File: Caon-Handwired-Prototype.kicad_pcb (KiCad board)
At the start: 6 copper layers, 27 parts, among them SW4 EC11 ENCODER 1, SW8 EC11 ENCODER 1, U1 74HC595, U2 74HC595, U3 SuperMini nRF52840

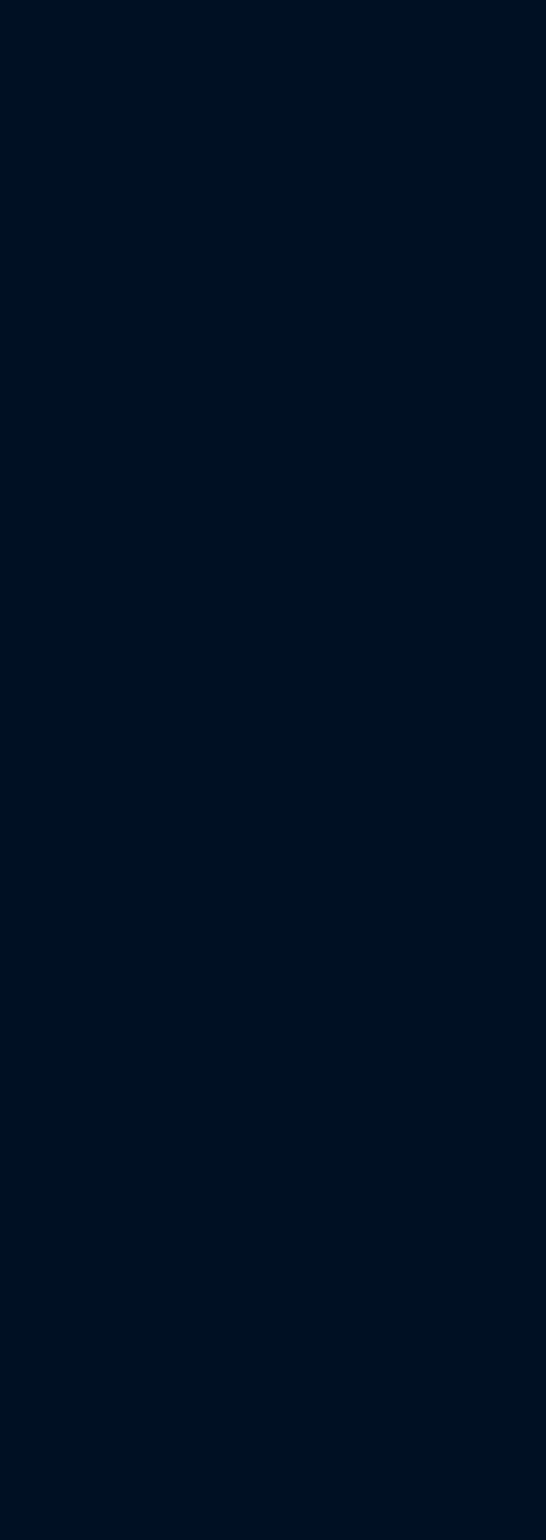
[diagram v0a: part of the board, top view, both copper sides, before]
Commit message: bump version to V0.1
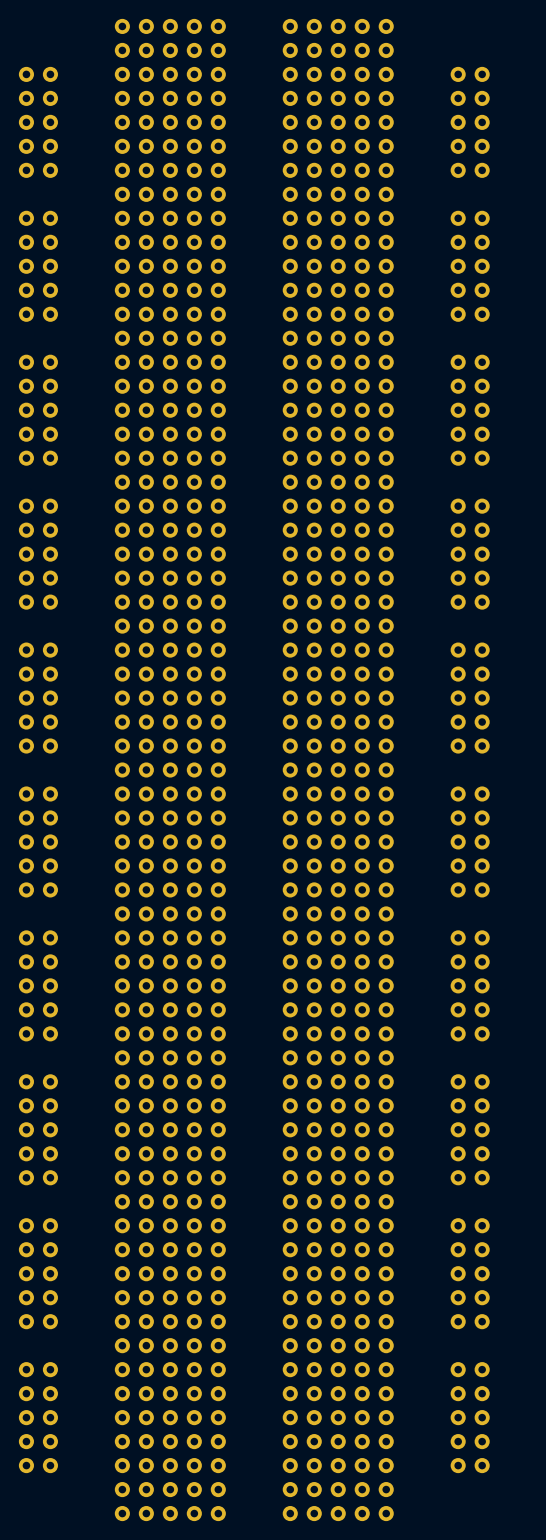
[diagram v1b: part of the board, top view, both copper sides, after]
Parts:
- added REF**: Standard 830 Breadboard, Caon_Footprint:Standard 830 Breadboard, F.Cu at (-17.8, 19.8)
